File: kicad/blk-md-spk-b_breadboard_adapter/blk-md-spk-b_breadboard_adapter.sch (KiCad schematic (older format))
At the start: 22 parts, among them J1 Jack_3.5mm_3pin, J2 Jack_3.5mm_3pin, P1 CONNECTOR, P2 CONNECTOR, U1 BLK-MD-SPK-B

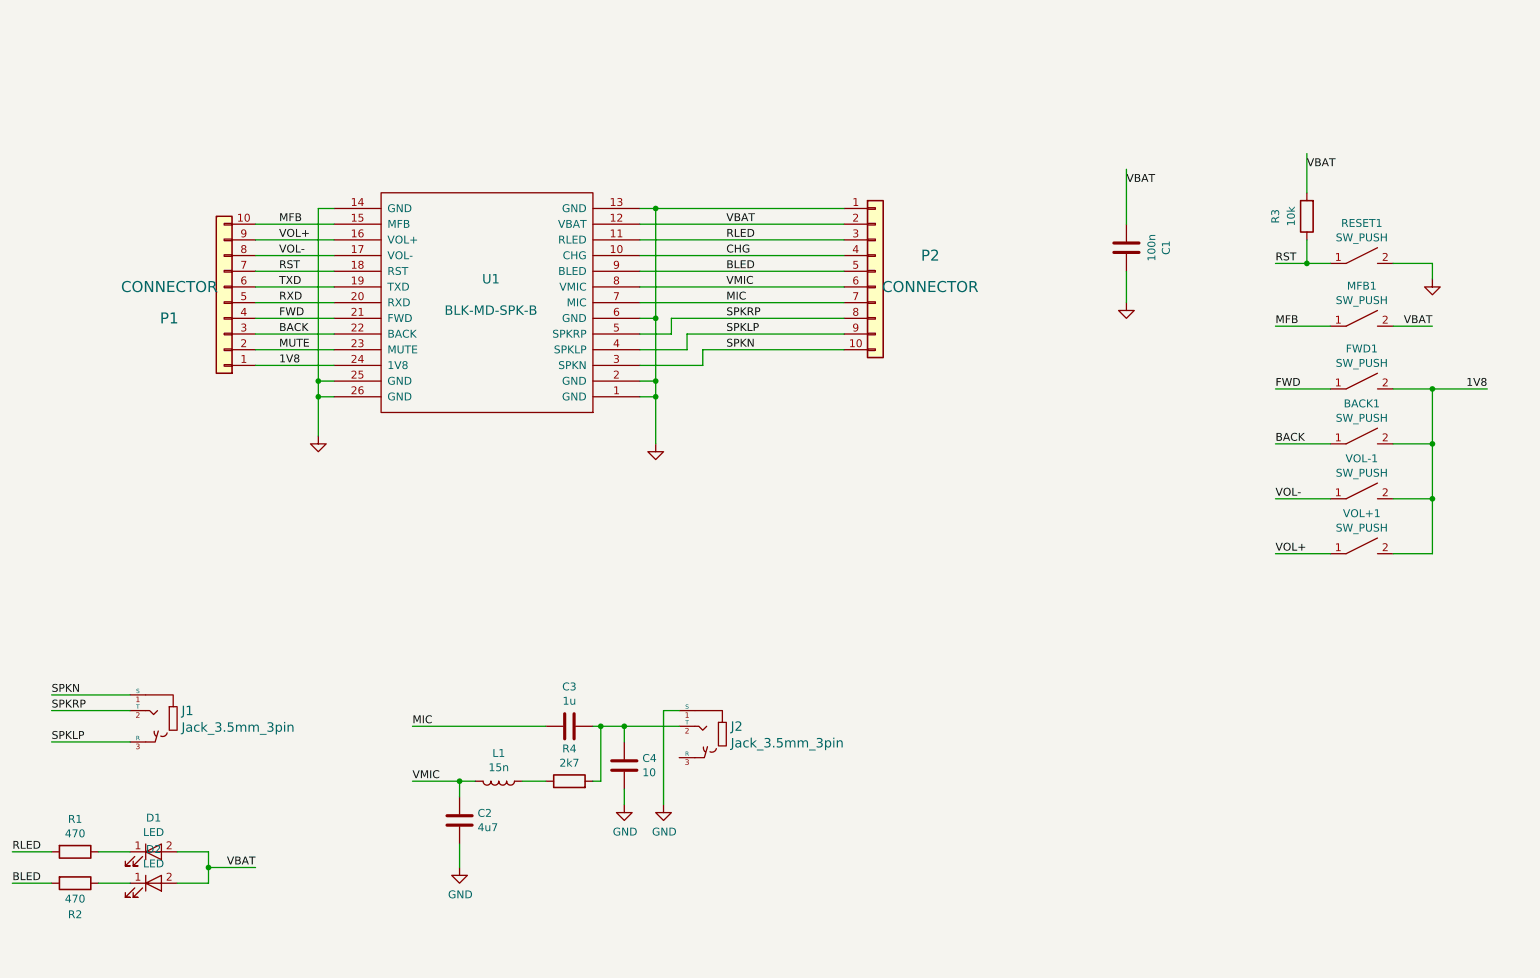
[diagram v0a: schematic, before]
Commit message: udpated to version 2.1
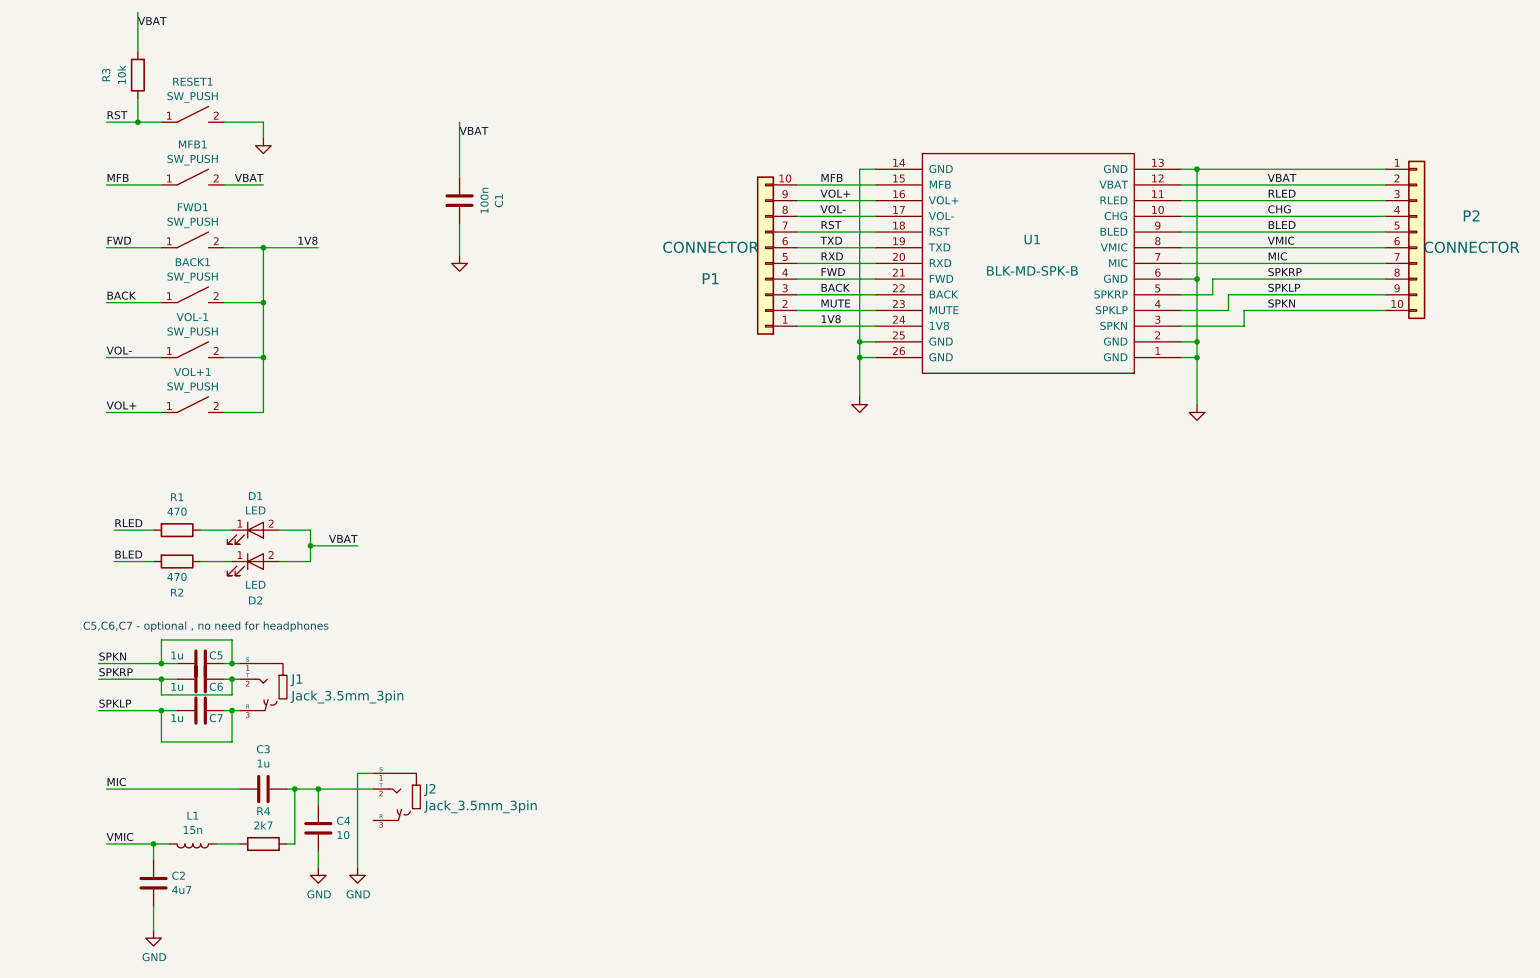
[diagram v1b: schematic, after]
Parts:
- added C5, C6, C7: 1u, Capacitors_SMD:C_1206_HandSoldering, symbol blk-md-spk-b_breadboard_adapter-rescue:C
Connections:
- net SPKLP: now also C7.1, C7.2
- net SPKN: now also C5.1, C5.2
- net SPKRP: now also C6.1, C6.2
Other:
- note added: "C5,C6,C7 - optional , no need for headphones"
- moved on the sheet: BACK1, C1, C2, C3, C4, D1, D2, FWD1, J1, J2, L1, MFB1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
